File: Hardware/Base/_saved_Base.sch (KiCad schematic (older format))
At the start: 8 parts

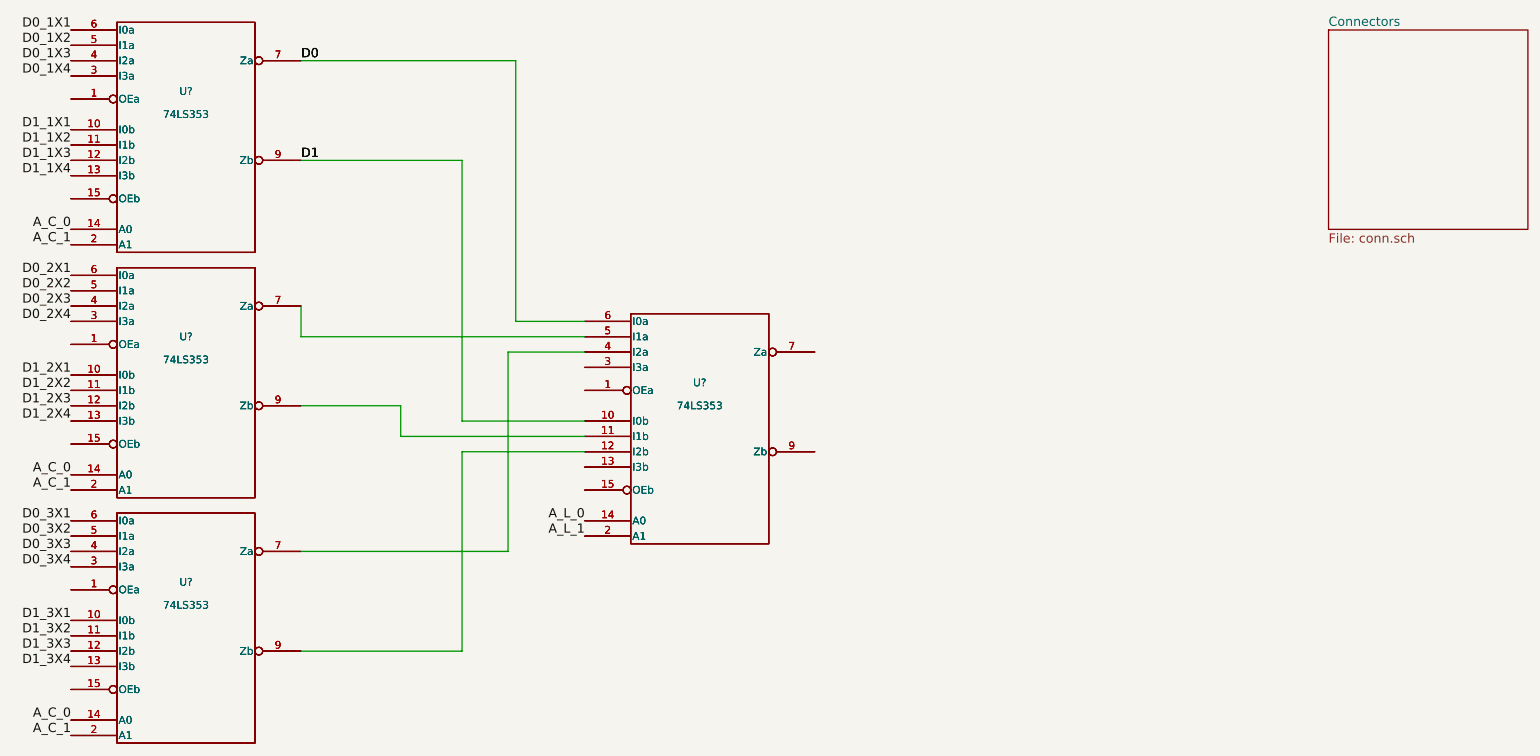
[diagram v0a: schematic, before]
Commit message: Base schematics almost done
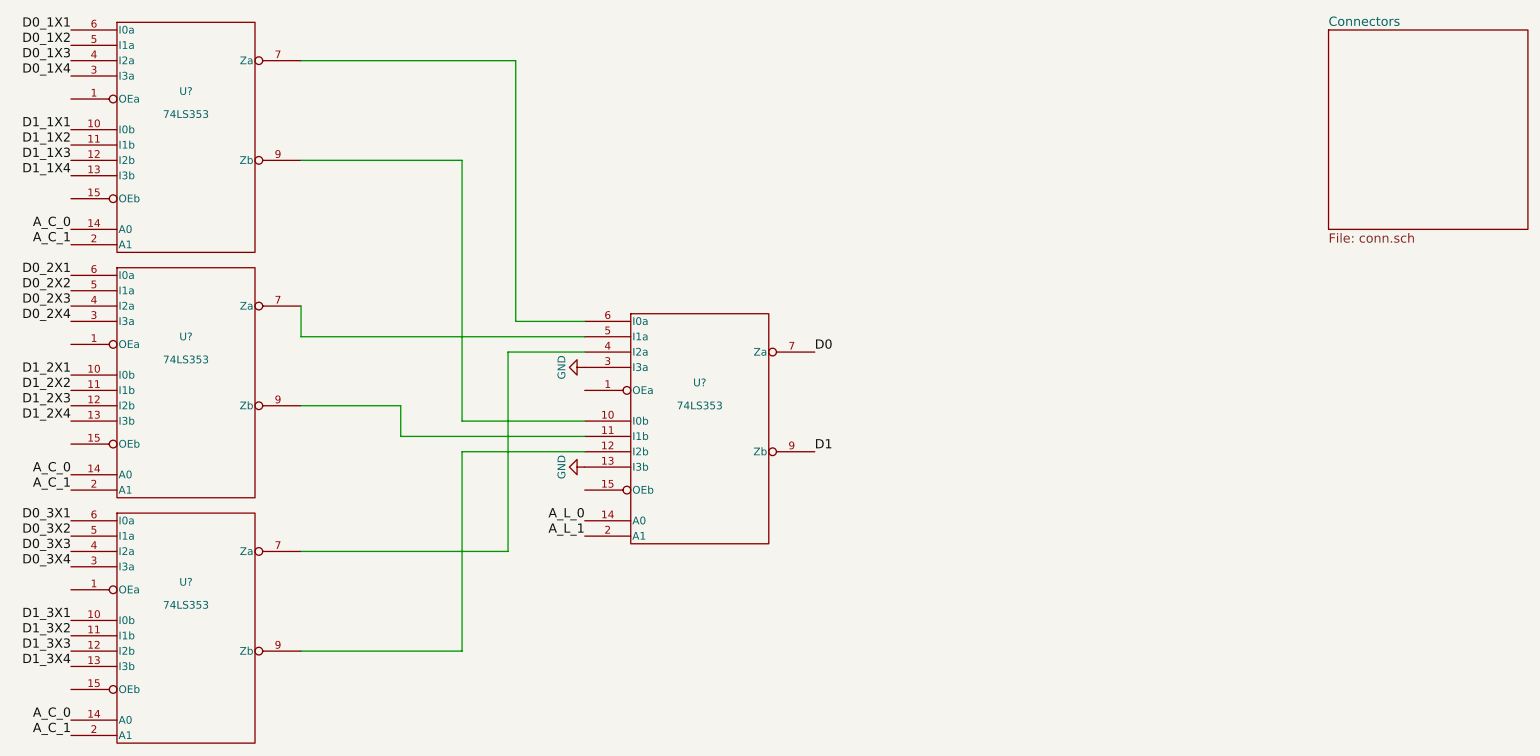
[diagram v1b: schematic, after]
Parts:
- removed U? (x4): 74LS353, symbol 74LS353
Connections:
- net D0: now also U?.7 (Za); no longer U?.6 (I0a), U?.7 (Za)
- net D1: now also U?.9 (Zb); no longer U?.10 (I0b), U?.9 (Zb)
- net GND: now also U?.13 (I3b), U?.3 (I3a)
- new net: U?.6 (I0a), U?.7 (Za)
- new net: U?.10 (I0b), U?.9 (Zb)
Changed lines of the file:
@@
 Comment4 ""
 $EndDescr
-$Comp
-L 74LS353 U?
-U 1 1 58EF2C3F
-P 2050 1550
-F 0 "U?" H 2050 1850 50  0000 C CNN
-F 1 "74LS353" H 2050 1700 50  0000 C CNN
-F 2 "" H 2050 1550 50  0000 C CNN
-F 3 "" H 2050 1550 50  0000 C CNN
-	1    2050 1550
-	1    0    0    -1
-$EndComp
-$Comp
-L 74LS353 U?
-U 1 1 58EF2C6E
-P 2050 3150
-F 0 "U?" H 2050 3450 50  0000 C CNN
-F 1 "74LS353" H 2050 3300 50  0000 C CNN
-F 2 "" H 2050 3150 50  0000 C CNN
-F 3 "" H 2050 3150 50  0000 C CNN
-	1    2050 3150
-	1    0    0    -1
-$EndComp
-$Comp
-L 74LS353 U?
-U 1 1 5901881A
-P 2050 4750
-F 0 "U?" H 2050 5050 50  0000 C CNN
-F 1 "74LS353" H 2050 4900 50  0000 C CNN
-F 2 "" H 2050 4750 50  0000 C CNN
-F 3 "" H 2050 4750 50  0000 C CNN
-	1    2050 4750
-	1    0    0    -1
-$EndComp
-Text Label 2800 1050 0    60   ~ 0
-D0
-Text Label 2800 1700 0    60   ~ 0
-D1
-$Comp
-L 74LS353 U?
-U 1 1 590190D3
-P 5400 3450
-F 0 "U?" H 5400 3750 50  0000 C CNN
-F 1 "74LS353" H 5400 3600 50  0000 C CNN
-F 2 "" H 5400 3450 50  0000 C CNN
-F 3 "" H 5400 3450 50  0000 C CNN
-	1    5400 3450
-	1    0    0    -1
-$EndComp
 Wire Wire Line
 	2800 1050 4200 1050
@@
 	1    0    0    -1
 $EndComp
-Text Label 2800 1050 0    60   ~ 0
-D0
-Text Label 2800 1700 0    60   ~ 0
-D1
 $Comp
 L 74LS353 U?
@@
 F1 "conn.sch" 60
 $EndSheet
-Text Label 1300 1500 2    60   ~ 0
-D1_1X1
 Text Label 1300 950  2    60   ~ 0
 D0_1X2
@@
 Text Label 1300 2250 2    60   ~ 0
 A_C_1
+Text Label 1300 1500 2    60   ~ 0
+D1_1X1
+Text Label 6150 2950 0    60   ~ 0
+D0
+Text Label 6150 3600 0    60   ~ 0
+D1
+$Comp
+L GND #PWR?
+U 1 1 590320A9
+P 4650 3050
+F 0 "#PWR?" H 4650 2800 50  0001 C CNN
+F 1 "GND" H 4650 2900 50  0000 C CNN
+F 2 "" H 4650 3050 50  0000 C CNN
+F 3 "" H 4650 3050 50  0000 C CNN
+	1    4650 3050
+	0    1    1    0
+$EndComp
+$Comp
+L GND #PWR?
+U 1 1 590320C5
+P 4650 3700
+F 0 "#PWR?" H 4650 3450 50  0001 C CNN
+F 1 "GND" H 4650 3550 50  0000 C CNN
+F 2 "" H 4650 3700 50  0000 C CNN
+F 3 "" H 4650 3700 50  0000 C CNN
+	1    4650 3700
+	0    1    1    0
+$EndComp
 $EndSCHEMATC
